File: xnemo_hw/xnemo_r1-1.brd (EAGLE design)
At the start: 39.8 x 31.3 mm, 36 parts, among them J1 MICRO_USB_B_RECEPT, J2 DM3D_MICRO_SD, J3 HEADER_2X5_0.05_SMD, J4 HEADER_2X5_0.05_THRU, J5 HEADER_2X5_0.05X0.1_SMD, U1 LTC3559, U2 L3GD20, U3 STM32F405RG, U5 HMC5883L, U6 ADXL345, X1 TXC_7A_XTAL

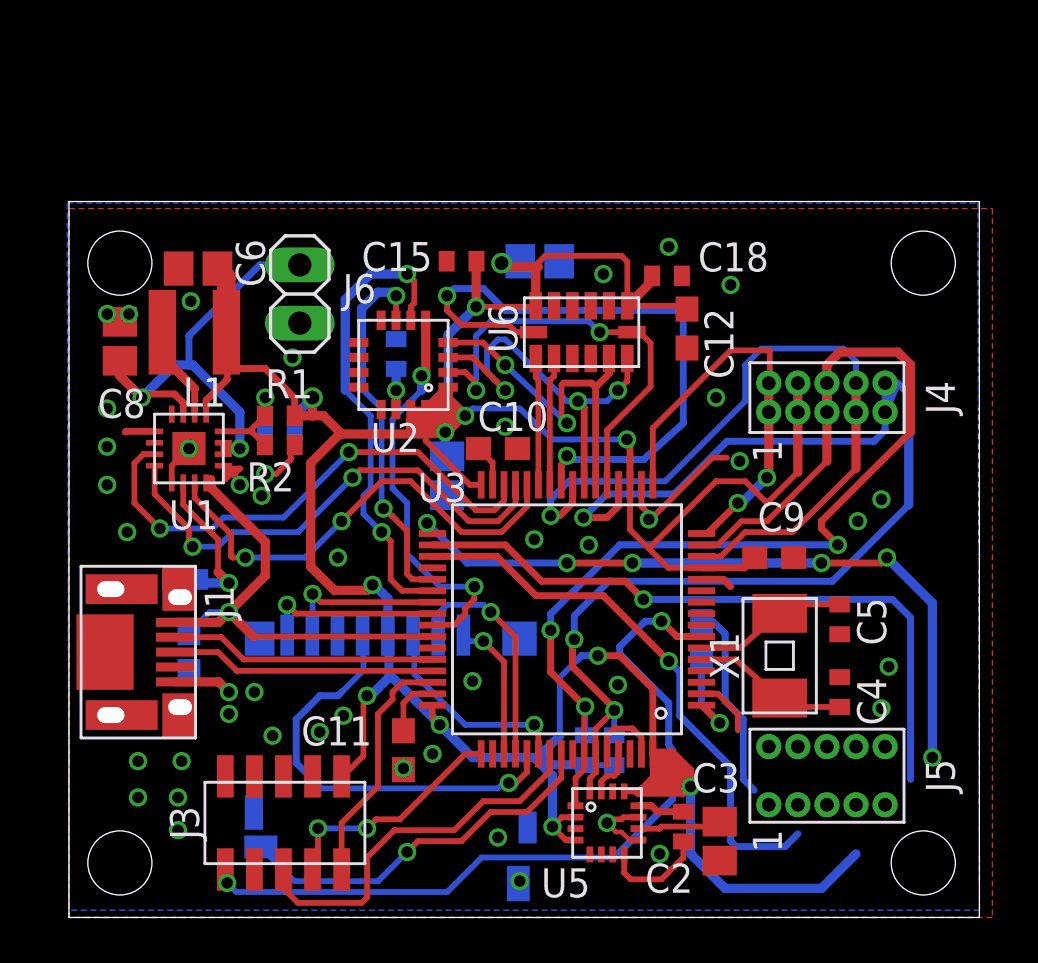
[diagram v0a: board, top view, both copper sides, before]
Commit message: I don't remember
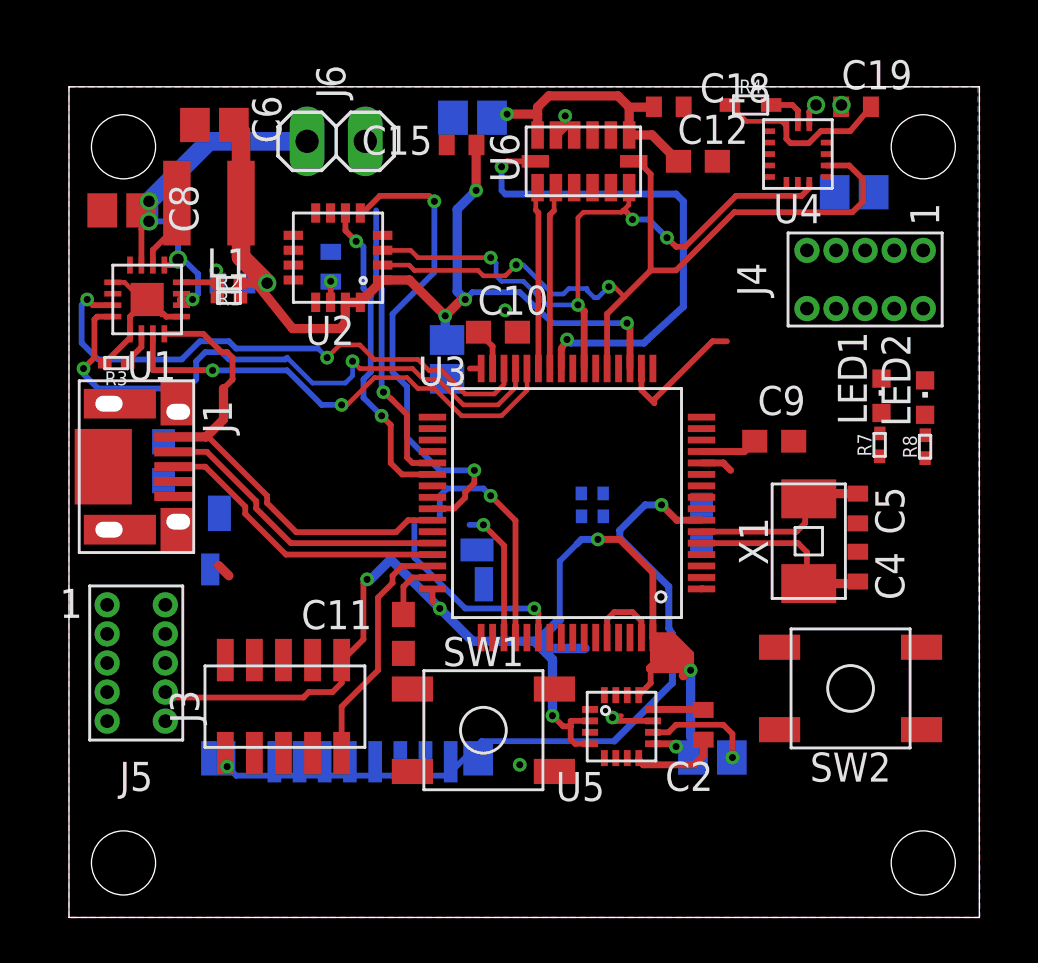
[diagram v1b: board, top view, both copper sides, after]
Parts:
- added C19: 100n, resistor:C0402
- added C20: 10u, resistor:C0805
- added LED1, LED2: (no value), led:CHIPLED_0603
- added R4: (no value), xnemo:SMD0603
- added R7, R8: (no value), xnemo:SMD0402
- added SW1, SW2: ALPS_SKQG, xnemo:ALPS_SKQG
- added U4: LPS331AP, xnemo:ST_HCLGA-16L
- C14: value 22p -> 10p
- J4: value HEADER_2X5_0.05_THRU -> HEADER_2X5_0.05X0.1_THRU; device xnemo:HEADER_2X5_0.05_THRU -> xnemo:HEADER_2X5_0.05X0.1_THRU
- J5: value HEADER_2X5_0.05X0.1_SMD -> HEADER_2X5_0.05X0.1_THRU
- R1, R2, R3, R5, R6: device resistor:R0402 -> xnemo:SMD0402
- moved J5 30.6 mm to (2.94, 11.1), turned to 0 degrees
- moved R5 10.7 mm to (23.3, 18.0)
- moved R6 10.7 mm to (22.4, 18.0)
- moved R3 9.92 mm to (2.06, 24.2), flipped to the top
- moved C7 8.41 mm to (4.13, 19.9)
- moved J1 8.10 mm to (1.75, 19.7)
- moved U6 7.46 mm to (22.5, 33.0)
- moved C18 7.38 mm to (26.2, 35.4)
- moved C12 7.32 mm to (27.5, 33.0), turned to 0 degrees
- moved C17 6.92 mm to (17.6, 34.9), turned to 0 degrees
- moved J6 6.85 mm to (11.7, 33.9), turned to 180 degrees
- moved R2 6.80 mm to (6.99, 27.1)
- moved U1 6.76 mm to (3.41, 27.0)
- moved C14 6.75 mm to (7.14, 27.7)
- moved J2 6.45 mm to (12.9, 12.8), turned to 0 degrees
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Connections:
- new net 3V3A: R4.P$2, U4.P$15
- new net N$2: LED1.A, R7.P$2
- new net N$3: LED2.A, R8.P$2
- new net PC14: R7.P$1, U3.P$3
- new net PC15: R8.P$1, U3.P$4
- new net SPI_CS_PRS: U4.P$8
- new net USER_BTN: SW2.1_1, U3.P$57
- net 3V3: now also C19.2, C20.1, R1.P$1, R4.P$1, R5.P$1, R6.P$1, U4.P$1, U4.P$14; no longer R1.2, R5.2, R6.2
- net BUCK_FB1: now also R1.P$2, R2.P$1; no longer R1.1, R2.2
- net GND: now also C19.1, C20.2, LED1.C, LED2.C, R2.P$2, R3.P$2, SW1.2_2, SW2.2_2, U4.P$10, U4.P$12, U4.P$13, U4.P$16, U4.P$5; no longer R2.1, R3.2
- net I2C_SCL: now also R6.P$2; no longer R6.1
- net I2C_SDA: now also R5.P$2; no longer R5.1
- net NRESET: now also SW1.1_2
- net POW_PROG: now also R3.P$1; no longer R3.1
- net SPI_CLK: now also U4.P$4
- net SPI_MISO: no longer U2.P$4, U6.P$12
- net SPI_MOSI: now also U4.P$6
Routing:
- net 3V3: track 178.7 -> 123.5 mm, vias 12 -> 11
- net I2C_SCL: track 40.2 -> 0.00 mm, vias 3 -> 0
- net I2C_SDA: track 33.5 -> 0.00 mm, vias 2 -> 0
- net PB12: track 31.2 -> 0.00 mm, vias 6 -> 0
- net PB13: track 29.3 -> 0.00 mm, vias 1 -> 0
- net PB14: track 24.5 -> 0.00 mm, vias 1 -> 0
- net PC4: track 22.1 -> 0.00 mm, vias 1 -> 0
- net PA4: track 19.5 -> 0.00 mm, vias 1 -> 0
- net SD_CLK: track 18.9 -> 0.00 mm, vias 1 -> 0
- net SWO: track 16.9 -> 0.00 mm
- net SD_DET: track 16.7 -> 0.00 mm, vias 1 -> 0
- net SPI_CLK: track 19.4 -> 35.8 mm
- net SPI_MISO: track 15.8 -> 0.00 mm, vias 2 -> 0
- net SPI_MOSI: track 17.7 -> 29.9 mm, vias 3 -> 4
- net PA0: track 12.1 -> 0.00 mm
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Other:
- board size 39.8 x 31.3 mm -> 39.8 x 36.3 mm
